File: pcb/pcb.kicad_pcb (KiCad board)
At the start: 2 copper layers, 117 x 96.2 mm, 49 parts, among them J1 BATT, J2 BATT, SW1 SW_SPST, SW10 SW_SPST, SW11 SW_SPST, SW12 SW_SPST, SW13 SW_SPST, SW14 SW_SPST, SW15 SW_SPST, SW16 SW_SPST, SW17 SW_SPST, SW18 SW_SPST, SW2 SW_SPST, SW3 SW_SPST, SW4 SW_SPST, SW5 SW_SPST, SW6 SW_SPST, SW7 SW_SPST, SW8 SW_SPST, SW9 SW_SPST, U1 XIAO_nRF52840

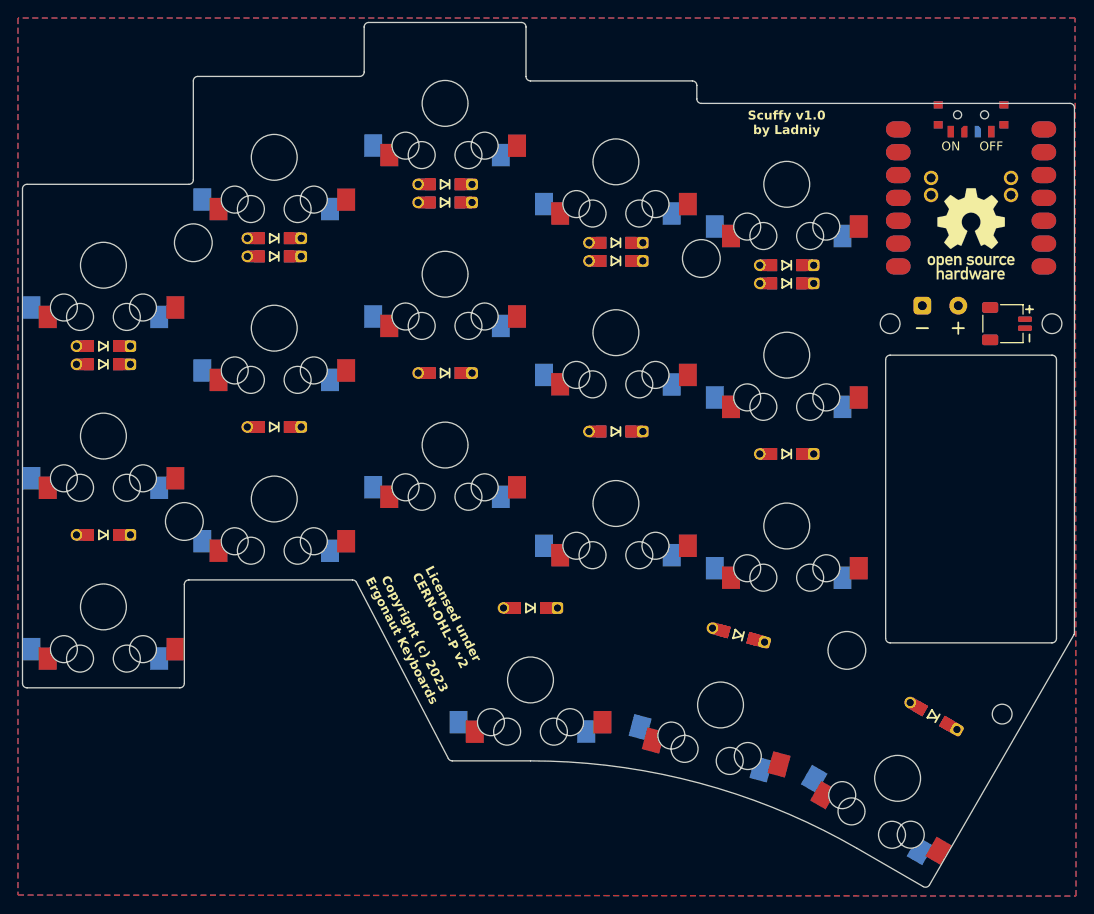
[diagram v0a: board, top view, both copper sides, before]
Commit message: feat: everything ready (no way)
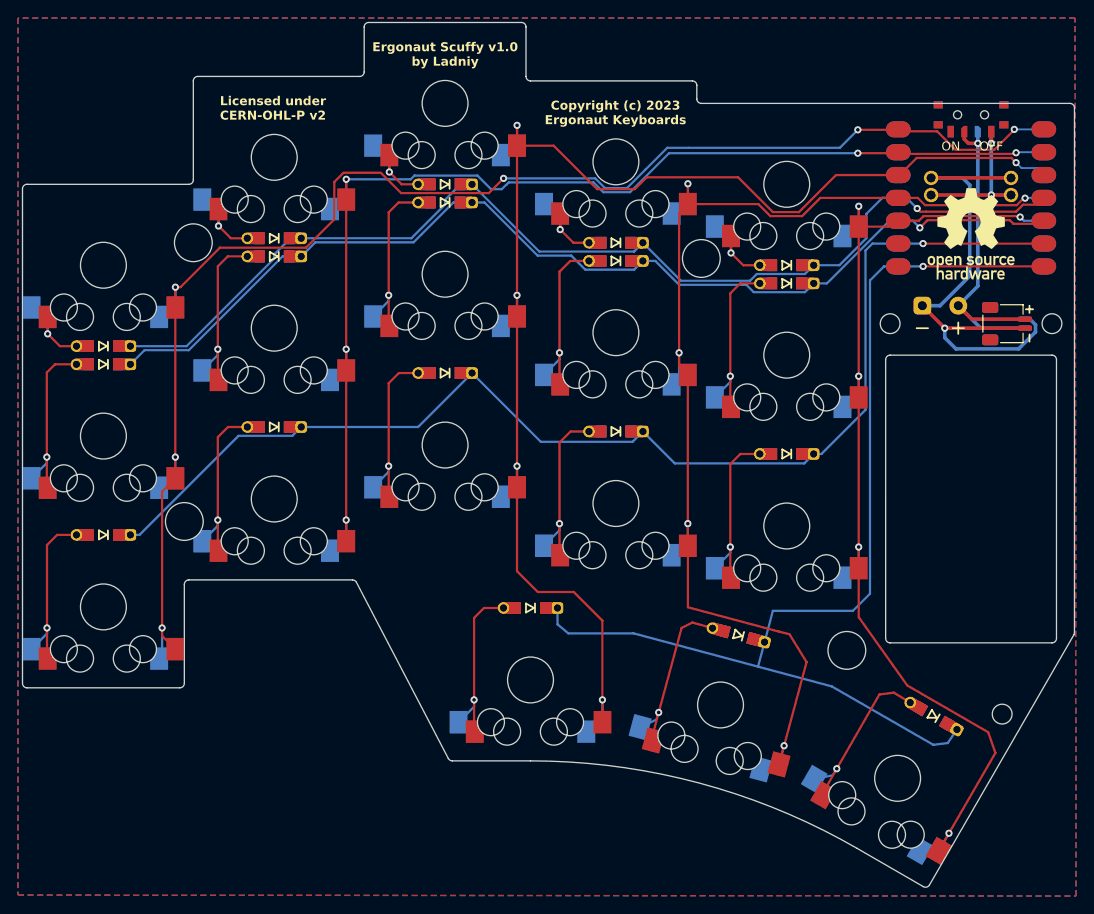
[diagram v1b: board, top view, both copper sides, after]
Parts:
- PWR1: moved to B.Cu
- turned PWR1 to 180 degrees
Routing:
- net C0: track 0.00 -> 164.7 mm, vias 0 -> 6
- net C2: track 0.00 -> 155.8 mm, vias 0 -> 5
- net R2: track 0.00 -> 135.2 mm, vias 0 -> 1
- net C1: track 0.00 -> 134.2 mm, vias 0 -> 5
- net C3: track 0.00 -> 133.5 mm, vias 0 -> 5
- net R3: track 0.00 -> 123.3 mm, vias 0 -> 1
- net R0: track 0.00 -> 122.0 mm, vias 0 -> 1
- net C4: track 0.00 -> 118.9 mm, vias 0 -> 5
- net R1: track 0.00 -> 118.7 mm, vias 0 -> 1
- net B-: track 0.00 -> 57.7 mm, vias 0 -> 1
- net Net-(J1-Pin_1): track 0.00 -> 39.3 mm, vias 0 -> 1
- net Net-(D16-A): track 0.00 -> 19.6 mm, vias 0 -> 1
- net Net-(D6-A): track 0.00 -> 19.6 mm, vias 0 -> 1
- net Net-(D18-A): track 0.00 -> 19.6 mm, vias 0 -> 1
- net Net-(D14-A): track 0.00 -> 19.5 mm, vias 0 -> 1
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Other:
- board text added: "Copyright (c) 2023 Ergonaut Keyboards"
- board text added: "Ergonaut Scuffy v1.0 by Ladniy"
- board text added: "Licensed under CERN-OHL-P v2"
- board text removed: "Licensed under CERN-OHL-P v2 Copyright (c) 2023 Ergonaut Keyboards"
- board text removed: "Scuffy v1.0 by Ladniy"

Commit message: feat: a lot of things, more in future pr
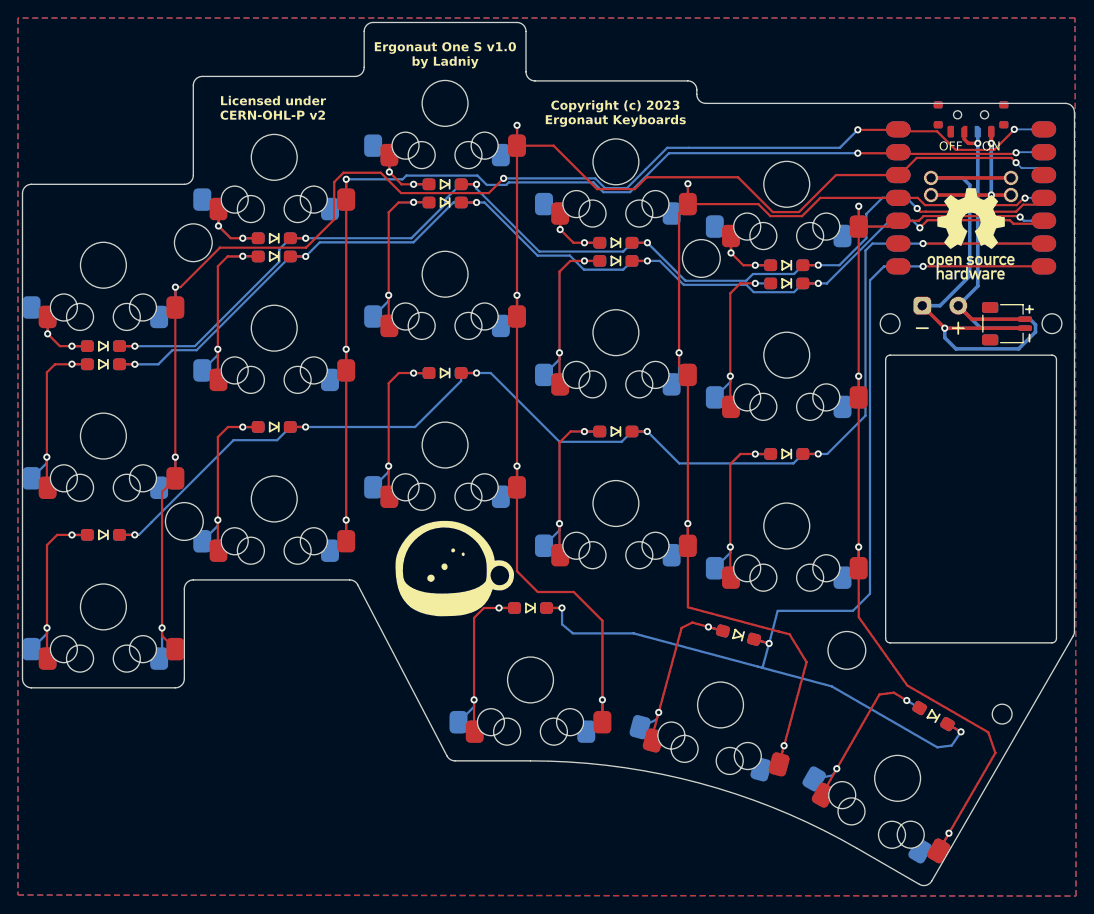
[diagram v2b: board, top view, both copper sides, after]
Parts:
- added G***: LOGO, one:en_logo, F.Cu at (131.9, 115.8)
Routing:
- net R2: track 135.2 -> 145.8 mm, vias 1 -> 6
- net R0: track 122.0 -> 132.6 mm, vias 1 -> 6
- net R3: track 123.3 -> 133.3 mm, vias 1 -> 4
- net R1: track 118.7 -> 128.6 mm, vias 1 -> 6
- net Net-(D8-A): track 19.5 -> 22.4 mm, vias 1 -> 2
- net Net-(D7-A): track 19.5 -> 22.4 mm, vias 1 -> 2
- net Net-(D6-A): track 19.6 -> 22.6 mm, vias 1 -> 2
- net Net-(D13-A): track 19.5 -> 22.4 mm, vias 1 -> 2
- net Net-(D15-A): track 19.5 -> 22.4 mm, vias 1 -> 2
- net Net-(D14-A): track 19.5 -> 22.5 mm, vias 1 -> 2
- net Net-(D12-A): track 19.5 -> 22.4 mm, vias 1 -> 2
- net Net-(D11-A): track 19.5 -> 22.4 mm, vias 1 -> 2
- net Net-(D5-A): track 9.33 -> 12.3 mm, vias 1 -> 2
- net Net-(D4-A): track 9.17 -> 12.1 mm, vias 1 -> 2
- net Net-(D1-A): track 9.33 -> 12.3 mm, vias 1 -> 2
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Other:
- board size 117 x 96.2 mm -> 117 x 96 mm
- board text added: "Ergonaut One S v1.0 by Ladniy"
- board text removed: "Ergonaut Scuffy v1.0 by Ladniy"
